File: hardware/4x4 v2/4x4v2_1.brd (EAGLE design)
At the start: 89.2 x 36.7 mm, 59 parts, among them IC1 PIC18F2480-I/SP, J1 USB1035-XX-X-X-X-B_REVE, T1 BC547, T2 BC547, T3 BC547, T4 BC547, U1 IR3315, U2 IR3315, U3 IR3315, U4 IR3315

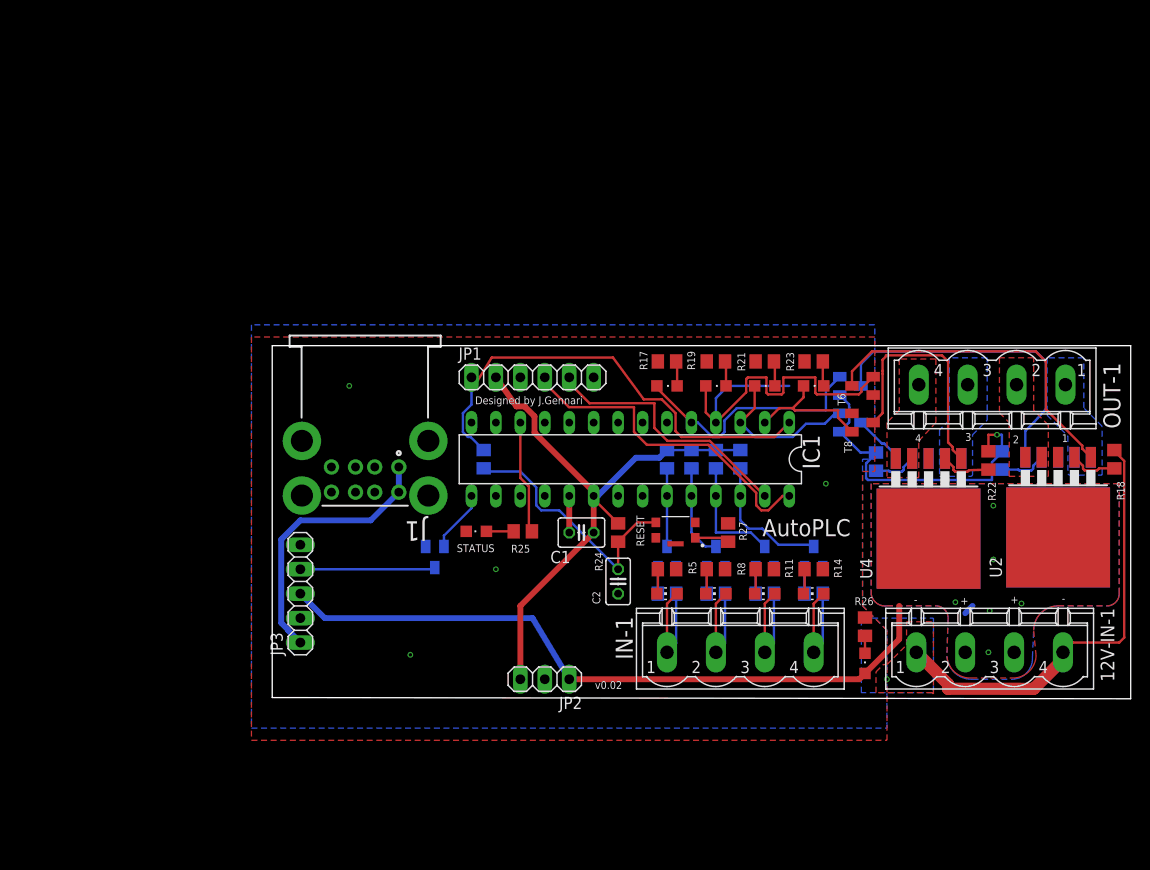
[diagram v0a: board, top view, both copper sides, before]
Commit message: Rev
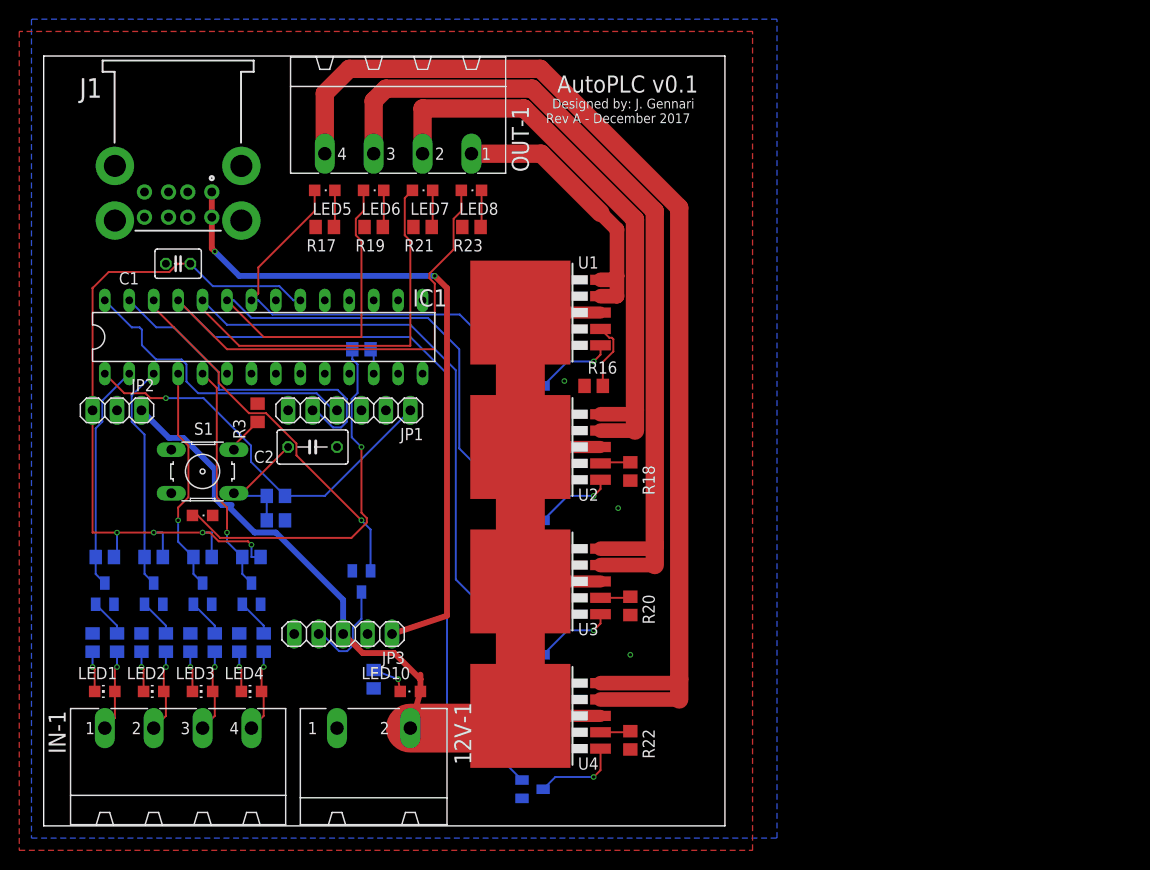
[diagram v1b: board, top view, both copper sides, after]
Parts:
- removed 12V-IN-1: MSTBV4, con-phoenix-508:MSTBV4
- removed R24: 10k, resistor:R0805
- removed R27: 100R, resistor:R0805
- added 12V-1: GMSTBA2, con-phoenix-762:GMSTBA2
- added R1, R2: (no value), resistor:R0805
- C1: value 0.1uF -> (none)
- C2: value 100nF -> (none); device resistor:C025-025X050 -> resistor:C050-035X075
- IN-1, OUT-1: value MSTBV4 -> MSTBA4; device con-phoenix-508:MSTBV4 -> con-phoenix-508:MSTBA4
- JP1: value ICSP -> (none)
- JP2: value 5V REG -> (none)
- JP3: value 5V USB -> (none)
- R17, R19, R21, R23, R25: value 150R -> (none)
- R3: value 10k -> (none)
- S1: value KMR421GULCLFS -> (none); device KMR421GULCLFS:SW_KMR421GULCLFS -> switch-omron:B3F-10XX
- moved OUT-1 68.2 mm to (36.8, 74.9)
- moved R11 60.2 mm to (15.2, 19.1), flipped to the bottom, turned to 90 degrees
- moved R14 60.2 mm to (20.3, 19.1), flipped to the bottom, turned to 90 degrees
- moved R5 60.2 mm to (5.08, 19.1), flipped to the bottom, turned to 90 degrees
- moved R8 60.2 mm to (10.2, 19.1), flipped to the bottom, turned to 90 degrees
- moved IN-1 59.8 mm to (14.0, 5.08)
- moved LED3 59.3 mm to (16.5, 14.0)
- moved LED4 59.3 mm to (21.6, 14.0)
- moved LED1 59.3 mm to (6.35, 14.0)
- moved LED2 59.3 mm to (11.4, 14.0)
- moved R6 59.3 mm to (6.35, 27.9), turned to 0 degrees
- moved T3 58.5 mm to (16.5, 24.1)
- moved T4 58.5 mm to (21.6, 24.1)
- moved T1 58.5 mm to (6.35, 24.1)
- moved T2 58.5 mm to (11.4, 24.1)
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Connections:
- new net 5V: JP1.2
- new net N$3: R2.2
- net 12V-1: now also 12V-1.2, U1.3, U2.3, U3.3, U4.3; no longer 12V-IN-1.2, 12V-IN-1.3
- net GND: now also 12V-1.1, R3.1; no longer 12V-IN-1.1, 12V-IN-1.4, R27.1, S1.5
- net MCLR: now also R1.1; no longer R3.1
- net N$1: now also R1.2, R2.1, S1.1; no longer R24.1, R3.2, S1.3
- net N$2: now also R3.2, S1.3; no longer R27.2, S1.1
- net SIGIN-1-1: now also IC1.2; no longer IC1.23
- net SIGIN-1-2: now also IC1.3; no longer IC1.24
- net SIGIN-1-3: now also IC1.4; no longer IC1.25
- net SIGIN-1-4: now also IC1.5; no longer IC1.26
- net SIGOUT-1-1: now also IC1.22; no longer IC1.5
- net SIGOUT-1-2: now also IC1.23; no longer IC1.4
- net SIGOUT-1-3: now also IC1.24; no longer IC1.3
- net SIGOUT-1-4: now also IC1.25; no longer IC1.2
- net SIGOUT-1-5: now also IC1.26; no longer IC1.15
- net VCC: no longer JP1.2, R24.2
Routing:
- net OUT-1-4: track 0.00 -> 118.0 mm
- net SIGOUT-1-4: track 13.9 -> 123.4 mm
- net OUT-1-3: track 0.00 -> 89.0 mm
- net SIGOUT-1-3: track 16.4 -> 101.6 mm
- net GND: track 84.0 -> 0.00 mm, vias 6 -> 3
- net 12V-1: track 73.1 -> 141.6 mm, vias 6 -> 0
- net OUT-1-2: track 0.00 -> 61.1 mm
- net OUT-1-5: track 28.4 -> 72.1 mm, vias 0 -> 2
- net SIGOUT-1-2: track 40.0 -> 77.1 mm
- net N$24: track 2.83 -> 38.9 mm, vias 0 -> 1
- net SIGOUT-1-5: track 6.43 -> 38.5 mm, vias 0 -> 1
- net OUT-1-1: track 0.00 -> 28.9 mm
- net N$15: track 34.8 -> 8.27 mm, vias 0 -> 1
- net N$12: track 33.3 -> 8.27 mm, vias 0 -> 1
- net SIGOUT-1-1: track 26.0 -> 45.6 mm
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- removed copper zone on layer 1, net 12V-1
- removed copper zone on layer 16, net 12V-1
- removed copper zone on layer 16, net OUT-1-1
- removed copper zone on layer 1, net OUT-1-2
- removed copper zone on layer 16, net OUT-1-3
- removed copper zone on layer 1, net OUT-1-4
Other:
- board size 89.2 x 36.7 mm -> 70.8 x 80 mm
- board text added: "AutoPLC v0.1"
- board text added: "Designed by: J. Gennari"
- board text added: "Rev A - December 2017"
- board text removed: "+"
- board text removed: "-"
- board text removed: "1"
- board text removed: "2"
- board text removed: "3"
- board text removed: "4"
- board text removed: "AutoPLC"
- board text removed: "Designed by J.Gennari"
- board text removed: "RESET"
- board text removed: "STATUS"
- board text removed: "v0.02"
